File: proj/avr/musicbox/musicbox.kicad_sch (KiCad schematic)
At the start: 55 parts, among them J1 USB, J2 UPDI, J3 NiMh*2, J4 OUT1, J5 OUT1, Q1 AO3401A, SW1 SW, SW2 SW, U1 CH340E, U2 BQ25172, U3 ATtiny402-SS, U4 ATtiny1604-SS, U5 TPS613222ADBV, U6 CH213K, U7 CH213K, U8 alps-rk10j12e, U9 PAM8406D

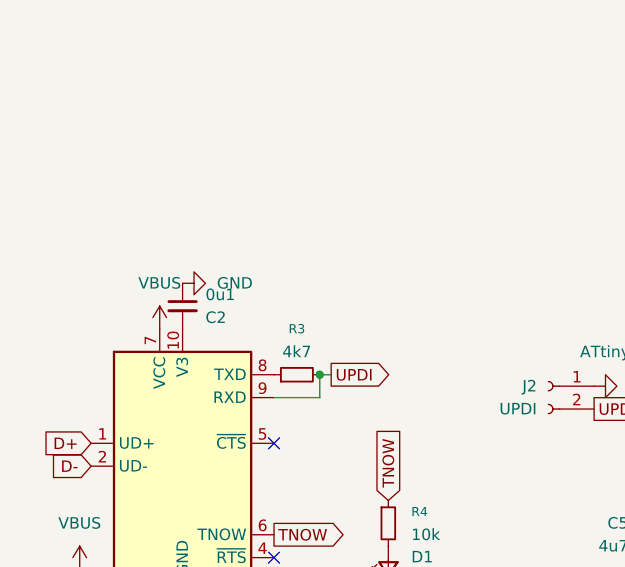
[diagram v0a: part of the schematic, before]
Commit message: -
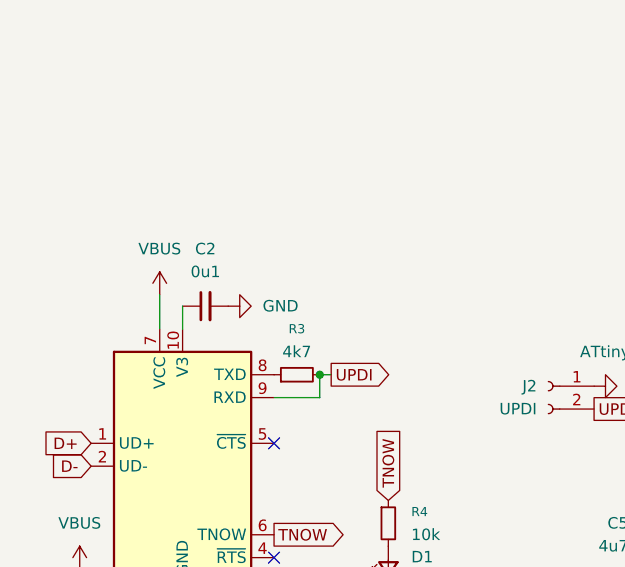
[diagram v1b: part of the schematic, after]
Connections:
- net GND: now also C2.2; no longer C2.1
- net at U1.10 (V3): now also C2.1; no longer C2.2
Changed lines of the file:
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@@
 	(wire
 		(pts
+			(xy 31.75 116.84) (xy 31.75 119.38)
+		)
+		(stroke
+			(width 0)
+			(type default)
+		)
+	)
+	(wire
+		(pts
 			(xy 135.89 148.59) (xy 149.86 148.59)
 		)
@@
 	(wire
 		(pts
+			(xy 29.21 115.57) (xy 29.21 119.38)
+		)
+		(stroke
+			(width 0)
+			(type default)
+		)
+	)
+	(wire
+		(pts
 			(xy 149.86 142.24) (xy 149.86 140.97)
 		)
@@
 	(symbol
 		(lib_id "power:VBUS")
-		(at 29.21 119.38 0)
+		(at 29.21 115.57 0)
 		(unit 1)
 		(exclude_from_sim no)
@@
 		(fields_autoplaced yes)
 		(property "Reference" "#PWR05"
-			(at 29.21 123.19 0)
+			(at 29.21 119.38 0)
 			(effects
 				(font
@@
 		)
 		(property "Value" "VBUS"
-			(at 29.21 114.3 0)
+			(at 29.21 110.49 0)
 			(effects
 				(font
@@
 		)
 		(property "Footprint" ""
-			(at 29.21 119.38 0)
+			(at 29.21 115.57 0)
 			(effects
 				(font
@@
 		)
 		(property "Datasheet" ""
-			(at 29.21 119.38 0)
+			(at 29.21 115.57 0)
 			(effects
 				(font
@@
 		)
 		(property "Description" "Power symbol creates a global label with name \"VBUS\""
-			(at 29.21 119.38 0)
+			(at 29.21 115.57 0)
 			(effects
 				(font
@@
 	(symbol
 		(lib_id "Device:C_Small")
+		(at 34.29 116.84 90)
+		(unit 1)
+		(exclude_from_sim no)
+		(in_bom yes)
+		(on_board yes)
+		(dnp no)
+		(fields_autoplaced yes)
+		(property "Reference" "C2"
+			(at 34.2963 110.49 90)
+			(effects
+				(font
+					(size 1.27 1.27)
+				)
+			)
+		)
+		(property "Value" "0u1"
+			(at 34.2963 113.03 90)
+			(effects
+				(font
+					(size 1.27 1.27)
+				)
+			)
+		)
+		(property "Footprint" "Capacitor_SMD:C_0603_1608Metric"
+			(at 34.29 116.84 0)
+			(effects
+				(font
+					(size 1.27 1.27)
+				)
+				(hide yes)
+			)
+		)
+		(property "Datasheet" "~"
+			(at 34.29 116.84 0)
+			(effects
+				(font
+					(size 1.27 1.27)
+				)
+				(hide yes)
+			)
+		)
+		(property "Description" "Unpolarized capacitor, small symbol"
+			(at 34.29 116.84 0)
+			(effects
+				(font
+					(size 1.27 1.27)
+				)
+				(hide yes)
+			)
+		)
+		(pin "2"
+		)
+		(pin "1"
+		)
+		(instances
+			(project ""
+				(path "/450caee3-b68b-423d-a829-37eac74bf274"
+					(reference "C2")
+					(unit 1)
+				)
+			)
+		)
+	)
+	(symbol
+		(lib_id "Device:C_Small")
 		(at 162.56 148.59 90)
 		(mirror x)
@@
 	)
 	(symbol
-		(lib_id "Device:C_Small")
-		(at 31.75 116.84 0)
-		(mirror y)
-		(unit 1)
-		(exclude_from_sim no)
-		(in_bom yes)
-		(on_board yes)
-		(dnp no)
-		(property "Reference" "C2"
-			(at 34.29 118.1165 0)
-			(effects
-				(font
-					(size 1.27 1.27)
-				)
-				(justify right)
-			)
-		)
-		(property "Value" "0u1"
-			(at 34.29 115.5765 0)
-			(effects
-				(font
-					(size 1.27 1.27)
-				)
-				(justify right)
-			)
-		)
-		(property "Footprint" "Capacitor_SMD:C_0603_1608Metric"
-			(at 31.75 116.84 0)
-			(effects
-				(font
-					(size 1.27 1.27)
-				)
-				(hide yes)
-			)
-		)
-		(property "Datasheet" "~"
-			(at 31.75 116.84 0)
-			(effects
-				(font
-					(size 1.27 1.27)
-				)
-				(hide yes)
-			)
-		)
-		(property "Description" "Unpolarized capacitor, small symbol"
-			(at 31.75 116.84 0)
-			(effects
-				(font
-					(size 1.27 1.27)
-				)
-				(hide yes)
-			)
-		)
-		(pin "2"
-		)
-		(pin "1"
-		)
-		(instances
-			(project "musicbox"
-				(path "/450caee3-b68b-423d-a829-37eac74bf274"
-					(reference "C2")
-					(unit 1)
-				)
-			)
-		)
-	)
-	(symbol
 		(lib_id "power:VBUS")
 		(at 20.32 146.05 0)
@@
 	(symbol
 		(lib_id "power:GND")
-		(at 31.75 114.3 90)
+		(at 36.83 116.84 90)
 		(unit 1)
 		(exclude_from_sim no)
@@
 		(fields_autoplaced yes)
 		(property "Reference" "#PWR06"
-			(at 38.1 114.3 0)
+			(at 43.18 116.84 0)
 			(effects
 				(font
@@
 		)
 		(property "Value" "GND"
-			(at 35.56 114.2999 90)
+			(at 40.64 116.8399 90)
 			(effects
 				(font
@@
 		)
 		(property "Footprint" ""
-			(at 31.75 114.3 0)
+			(at 36.83 116.84 0)
 			(effects
 				(font
@@
 		)
 		(property "Datasheet" ""
-			(at 31.75 114.3 0)
+			(at 36.83 116.84 0)
 			(effects
 				(font
@@
 		)
 		(property "Description" "Power symbol creates a global label with name \"GND\" , ground"
-			(at 31.75 114.3 0)
+			(at 36.83 116.84 0)
 			(effects
 				(font

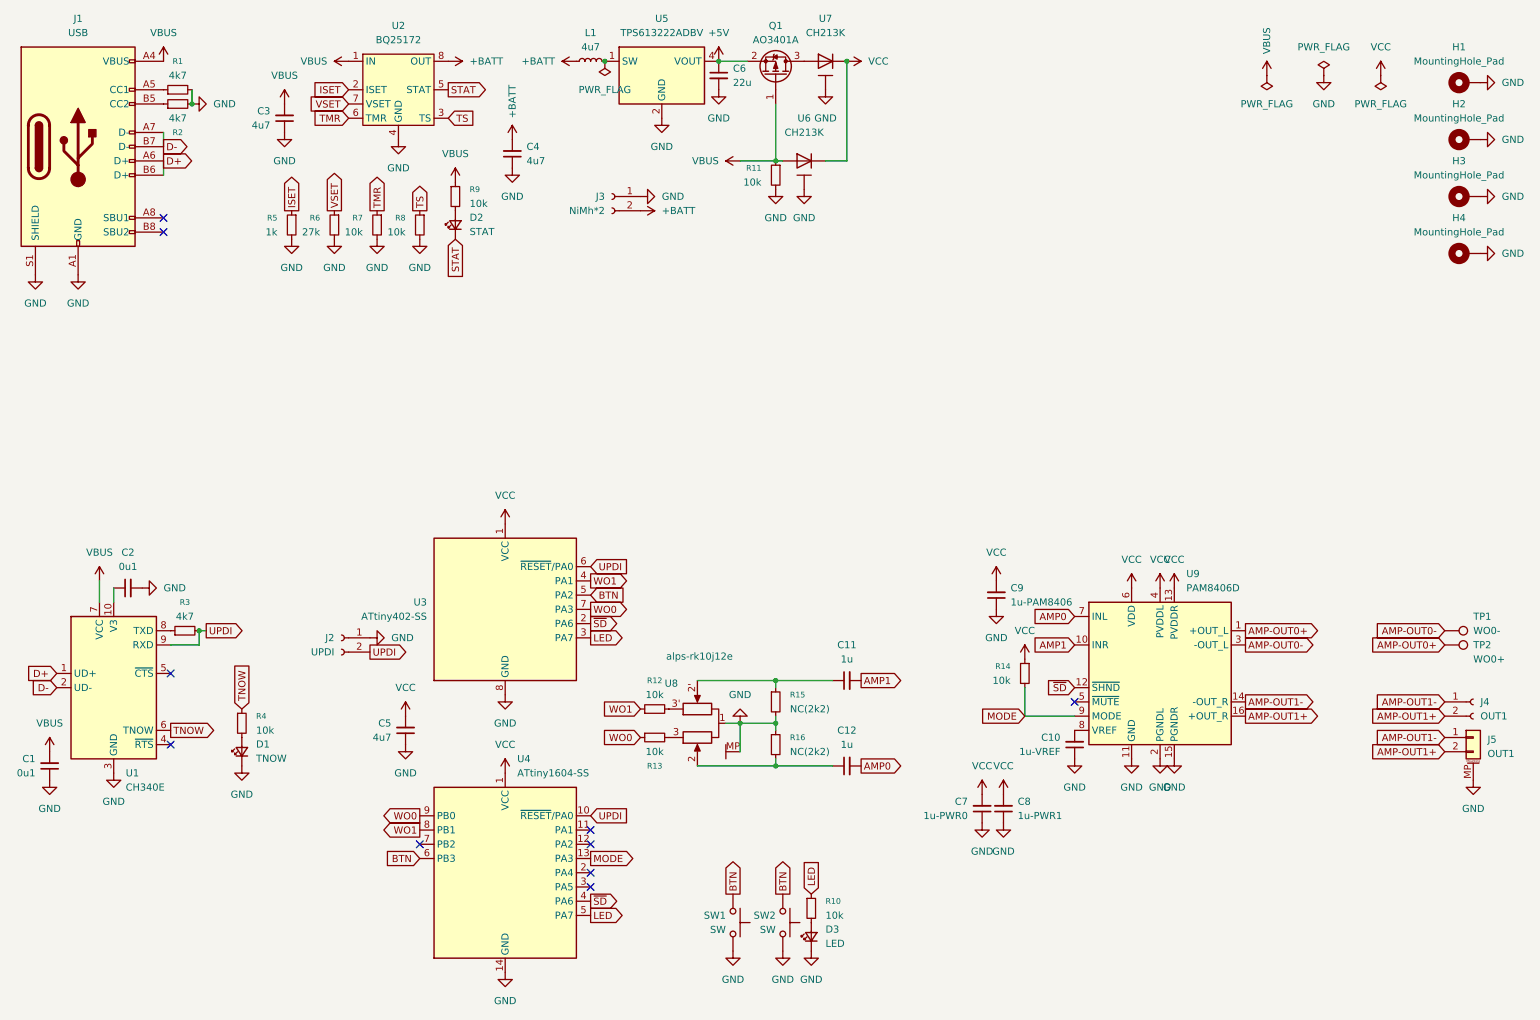
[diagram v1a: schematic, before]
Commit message: -
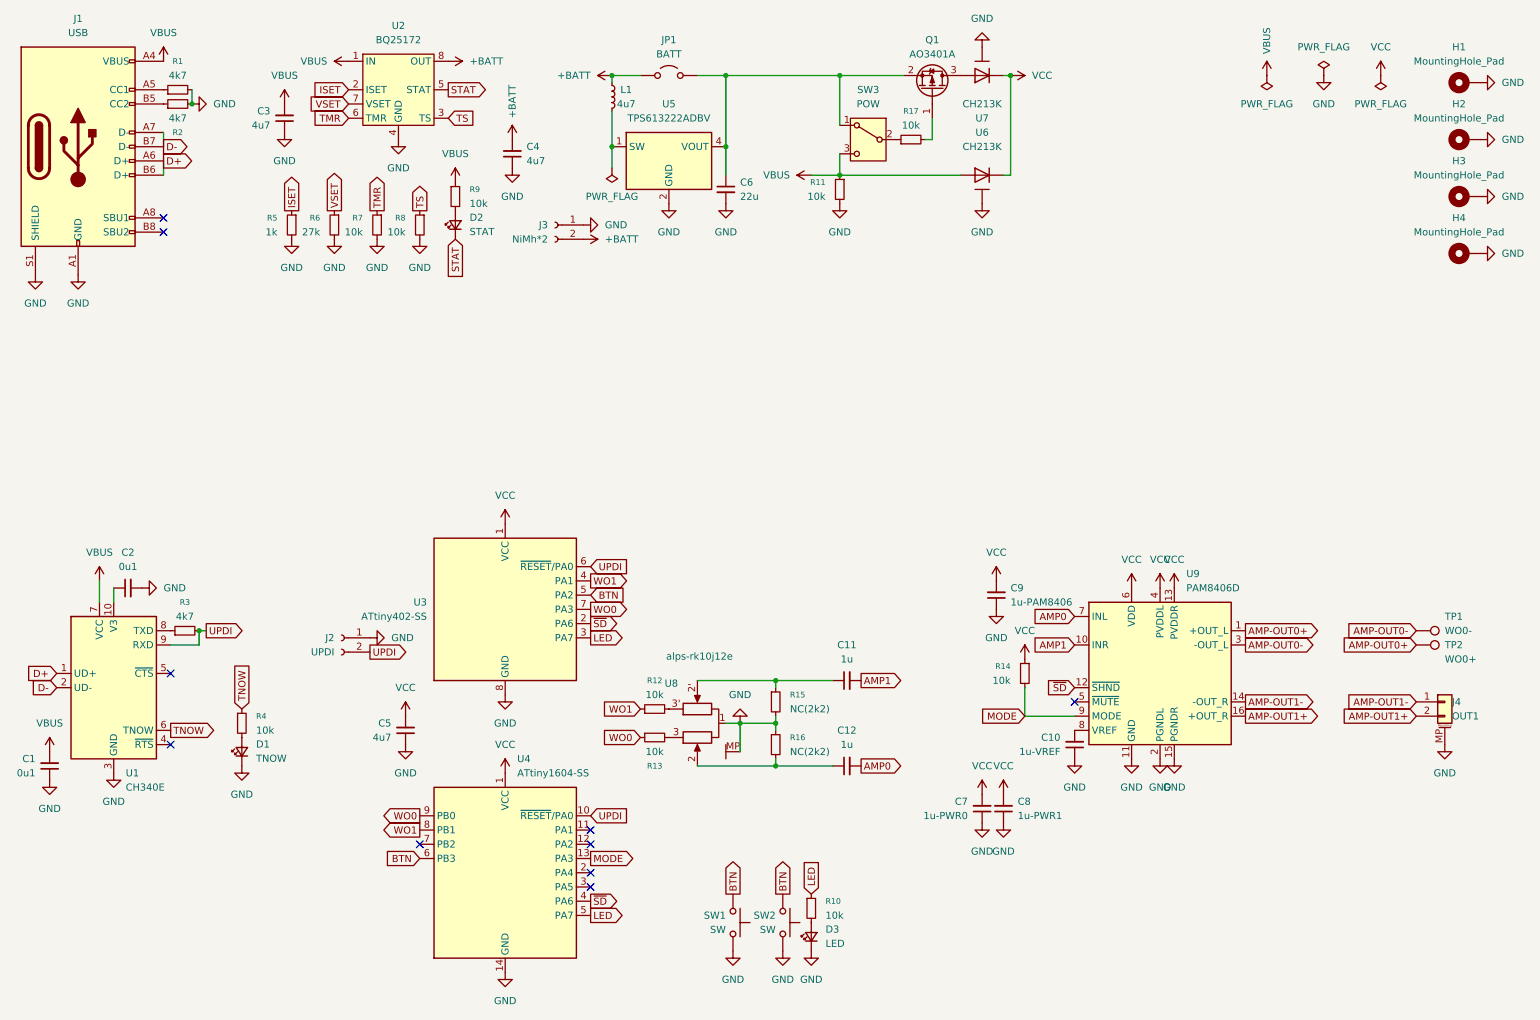
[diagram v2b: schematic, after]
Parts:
- removed J5: OUT1, Connector_JST:JST_ZH_S2B-ZR-SM4A-TF_1x02-1MP_P1.50mm_Horizontal, symbol Connector_Generic_MountingPin:Conn_01x02_MountingPin
- added JP1: BATT, Resistor_SMD:R_0603_1608Metric, symbol Jumper:Jumper_2_Open
- added R17: 10k, Resistor_SMD:R_0603_1608Metric, symbol Device:R_Small
- added SW3: POW, Library:IS-1245T-G, symbol Switch:SW_SPDT
- J4: footprint Connector_JST:JST_XH_S2B-XH-A_1x02_P2.50mm_Horizontal -> Connector_JST:JST_ZH_S2B-ZR-SM4A-TF_1x02-1MP_P1.50mm_Horizontal; symbol Connector:Conn_01x02_Socket -> Connector_Generic_MountingPin:Conn_01x02_MountingPin
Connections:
- net +BATT: now also JP1.1 (A)
- net GND: now also J4.MP (MountPin)
- net VBUS: now also SW3.3 (C); no longer Q1.1 (G)
- net +5V: no longer names the net of C6.1, Q1.2 (S), U5.4 (VOUT)
- net +5V: now also JP1.2 (B), SW3.1 (A)
- new net: R17.1, SW3.2 (B)
- new net: Q1.1 (G), R17.2
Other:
- moved on the sheet: C6, J3, L1, Q1, R11, TP1, TP2, U5, U6, U7
